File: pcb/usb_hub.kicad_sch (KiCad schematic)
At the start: 36 parts, among them J5 USB_C1_USB2.0, J6 USB_A1, J7 USB_A2, U2 USB2514-HZH (C184347), U3 TPS62140, U4 TPS2069C, U5 TPS2069C, U6 TPS2069C, Y1 48mhz

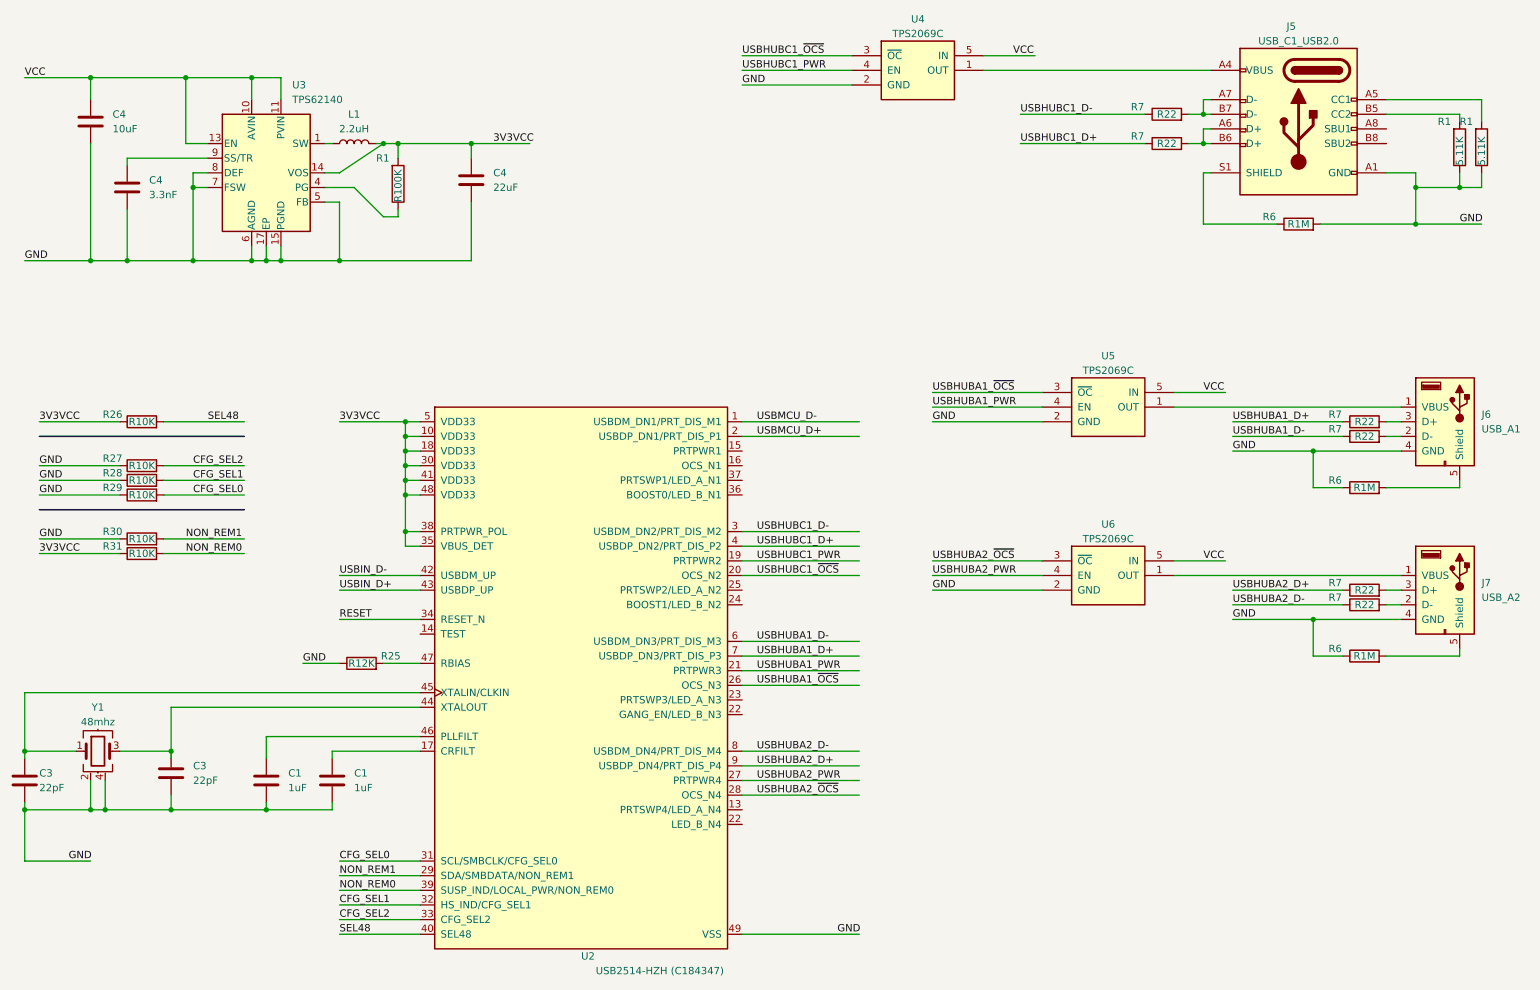
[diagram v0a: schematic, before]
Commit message: shematic and pcb update
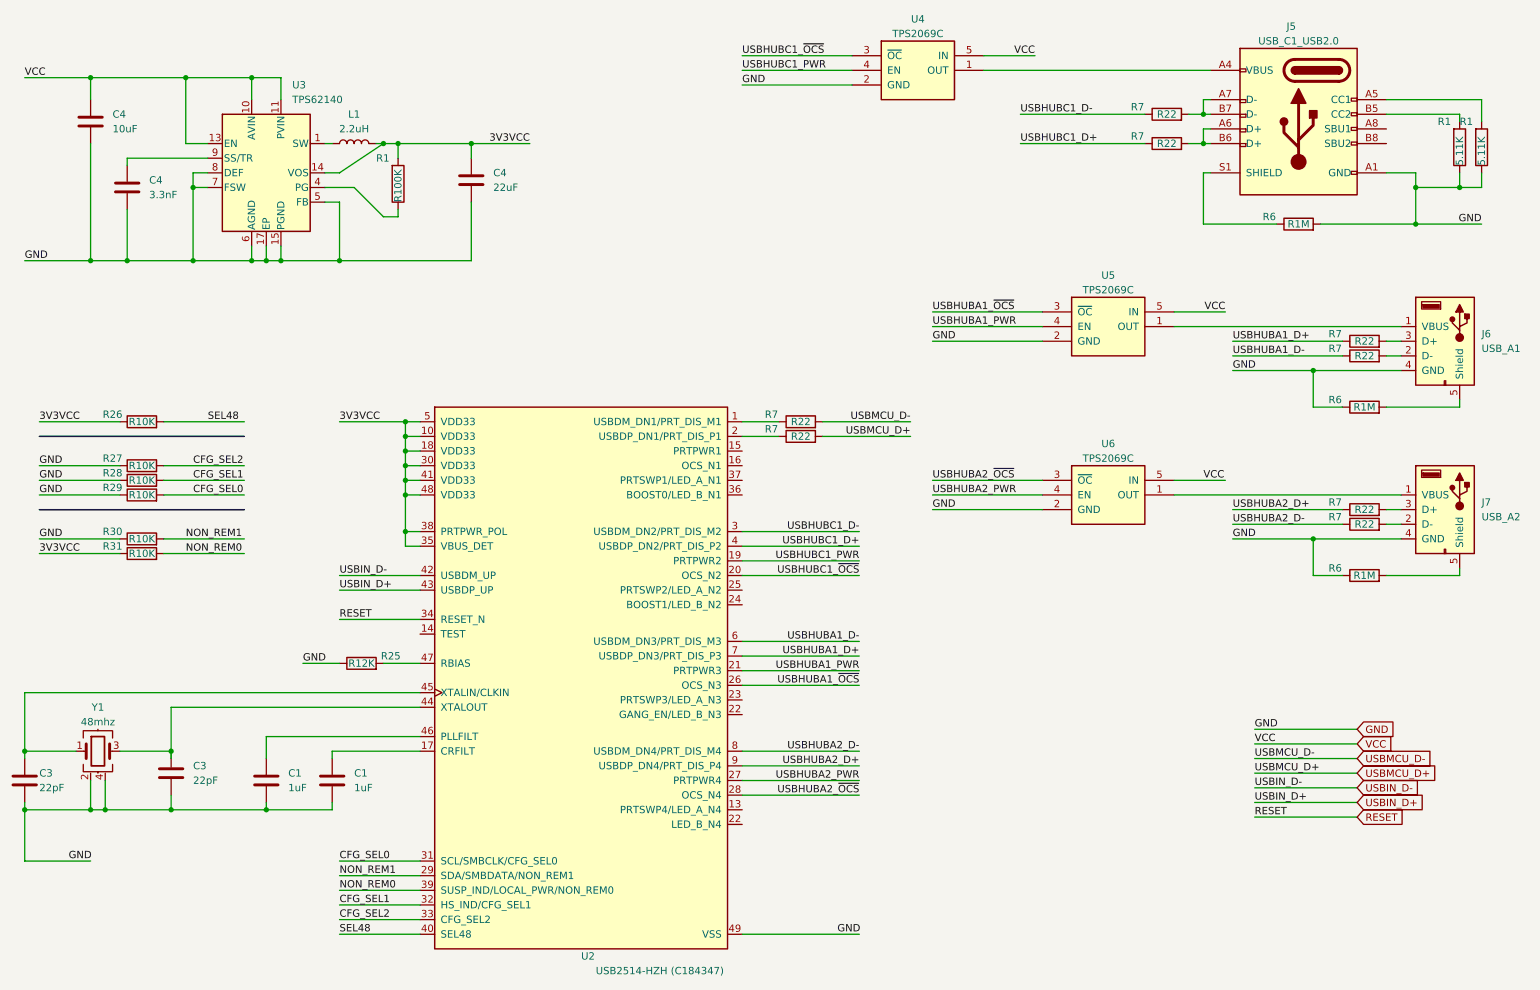
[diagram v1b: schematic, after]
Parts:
- added R7 (x2): R22, Resistor_SMD:R_0402_1005Metric, symbol Device:R
- J6, J7: footprint (none) -> NORMAL_USB_A:GT_USBA
- L1: footprint (none) -> Inductor_SMD:L_0805_2012Metric
- R25, R26, R27, R28, R29, R30, R31: footprint (none) -> Resistor_SMD:R_0402_1005Metric
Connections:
- net USBMCU_D+: now also R7.2; no longer U2.2 (USBDP_DN1/PRT_DIS_P1)
- net USBMCU_D-: now also R7.2; no longer U2.1 (USBDM_DN1/PRT_DIS_M1)
- new net: R7.1, U2.1 (USBDM_DN1/PRT_DIS_M1)
- new net: R7.1, U2.2 (USBDP_DN1/PRT_DIS_P1)
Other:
- moved on the sheet: J6, J7, R6, R7, U5, U6
